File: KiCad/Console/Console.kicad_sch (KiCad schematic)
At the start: 7 parts, among them J1 Conn_01x10_Pin, J2 Conn_01x08_Pin, J3 Conn_01x08_Pin, J4 Conn_01x06_Pin, J5 Conn_01x06, SW1 RotaryEncoder_Switch, U1 OLED SSD1306 128X64

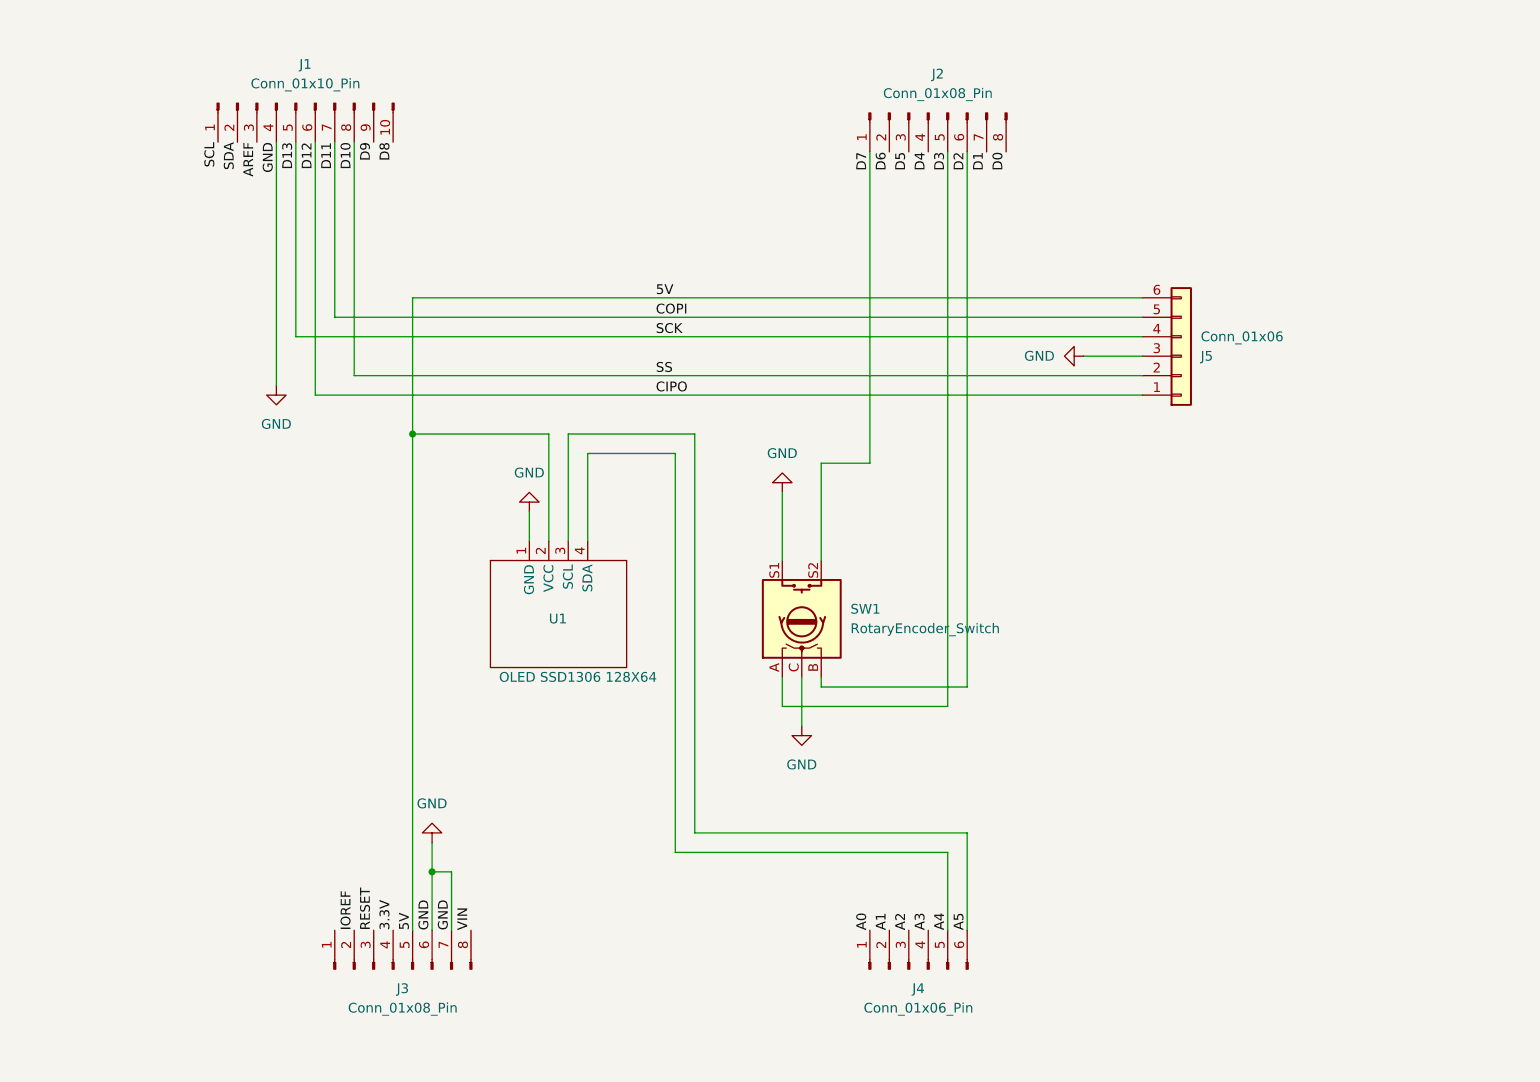
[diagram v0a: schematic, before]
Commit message: 測定フォルダ更新。
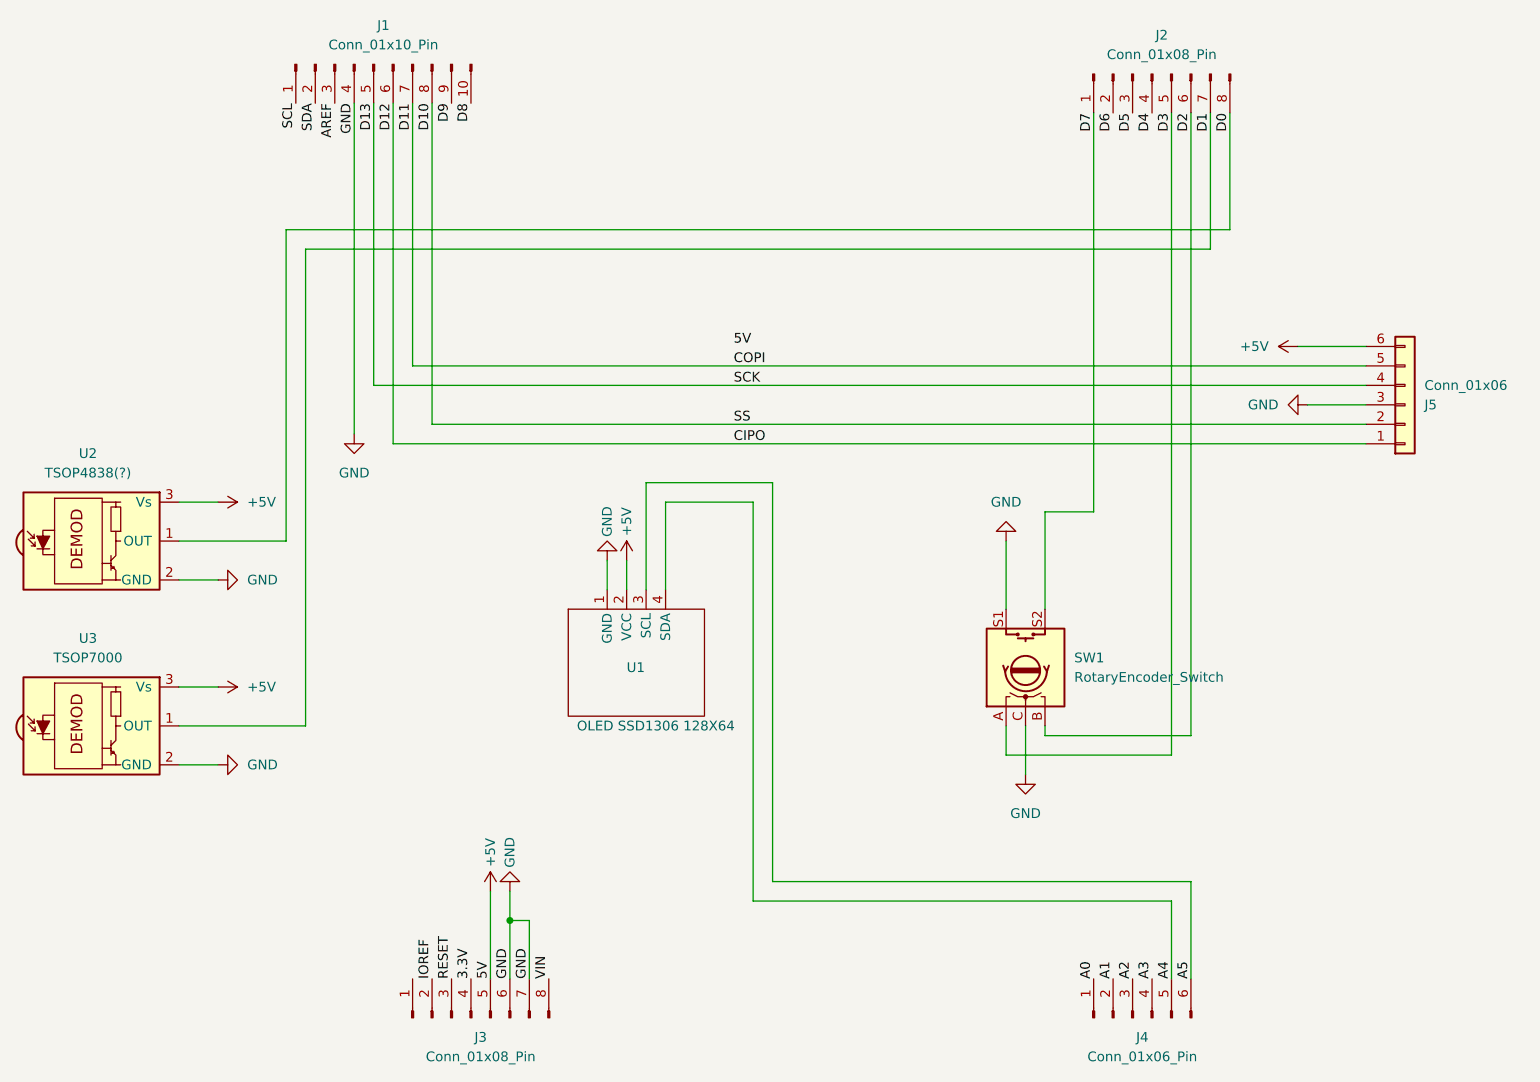
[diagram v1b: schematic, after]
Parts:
- added U2: TSOP4838(?), OptoDevice:Vishay_MOLD-3Pin, symbol Interface_Optical:TSOP41xx
- added U3: TSOP7000, OptoDevice:Vishay_MOLD-3Pin, symbol Interface_Optical:TSOP41xx
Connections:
- net D0: now also U2.1 (OUT)
- net D1: now also U3.1 (OUT)
- net GND: now also U2.2 (GND), U3.2 (GND)
- net 5V renamed +5V
- net +5V: now also U2.3 (Vs), U3.3 (Vs)
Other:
- moved on the sheet: J1, J2, J3, J4, J5, SW1, U1
